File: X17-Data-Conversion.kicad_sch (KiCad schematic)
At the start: 23 parts, among them J1 Conn_01x05, J2 BG030_-_-_-_6_-_-_X_-_XXX_-_-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, J3 BG030_-_-_-_6_-_-_X_-_XXX_-_-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, SW1 1825910-6, U1 ABLS-8.000MHZ-B2-T, U2 STM32F091CCTx, U5 AZ1117IH-3.3TRG1

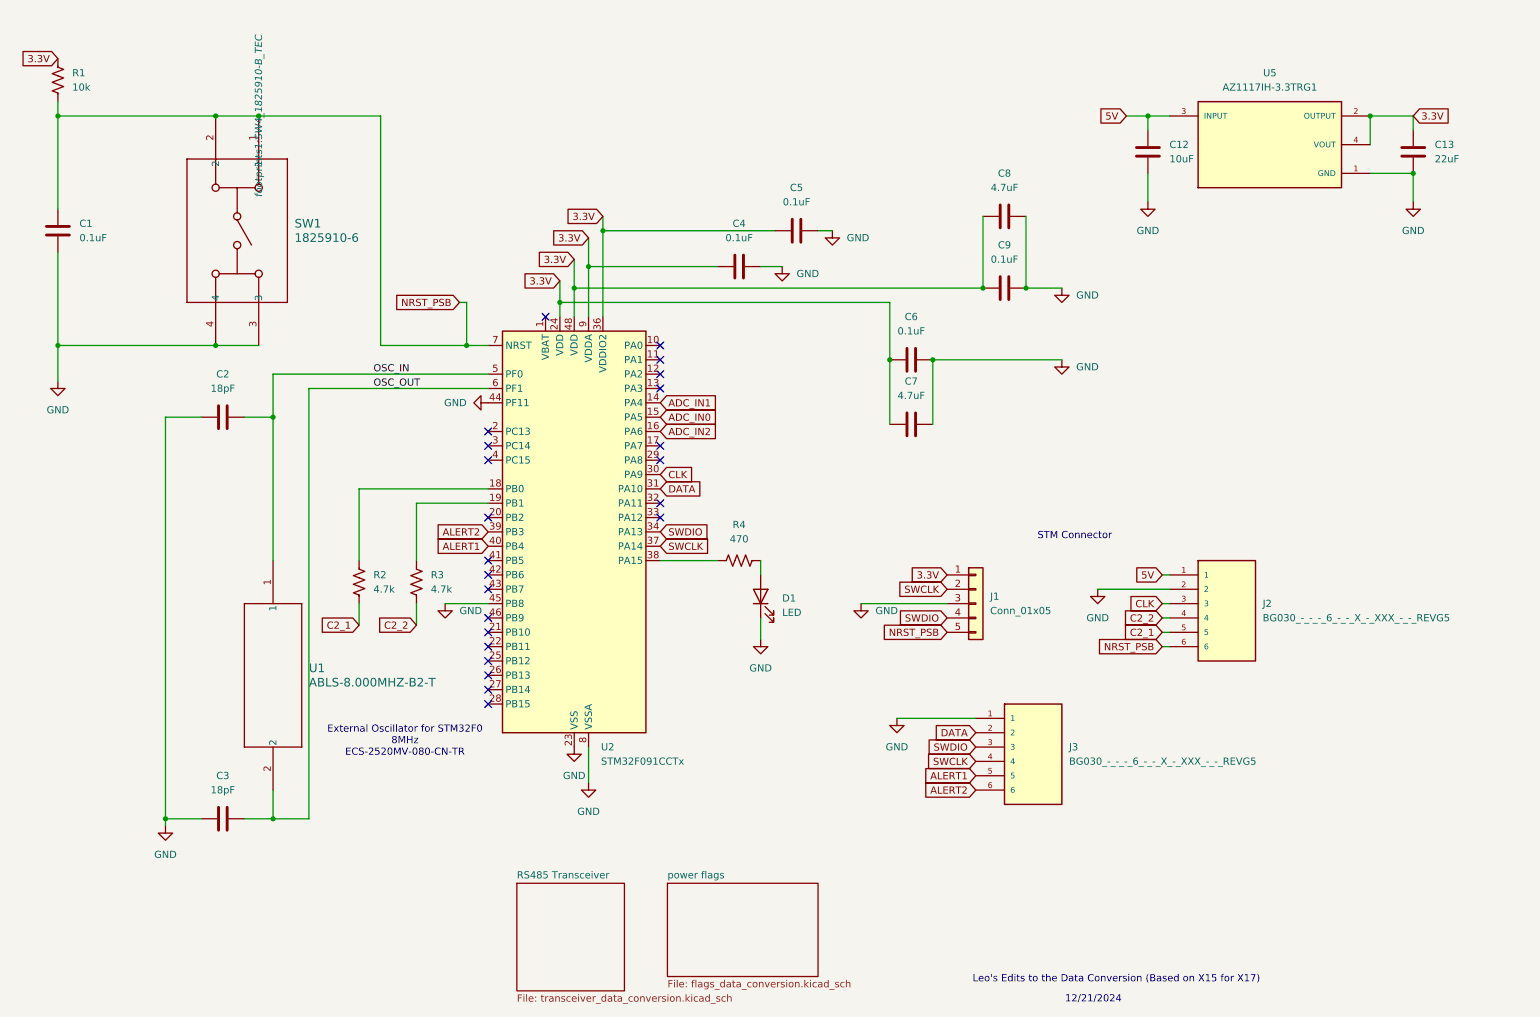
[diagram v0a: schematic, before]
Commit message: meeting today, need to rewire
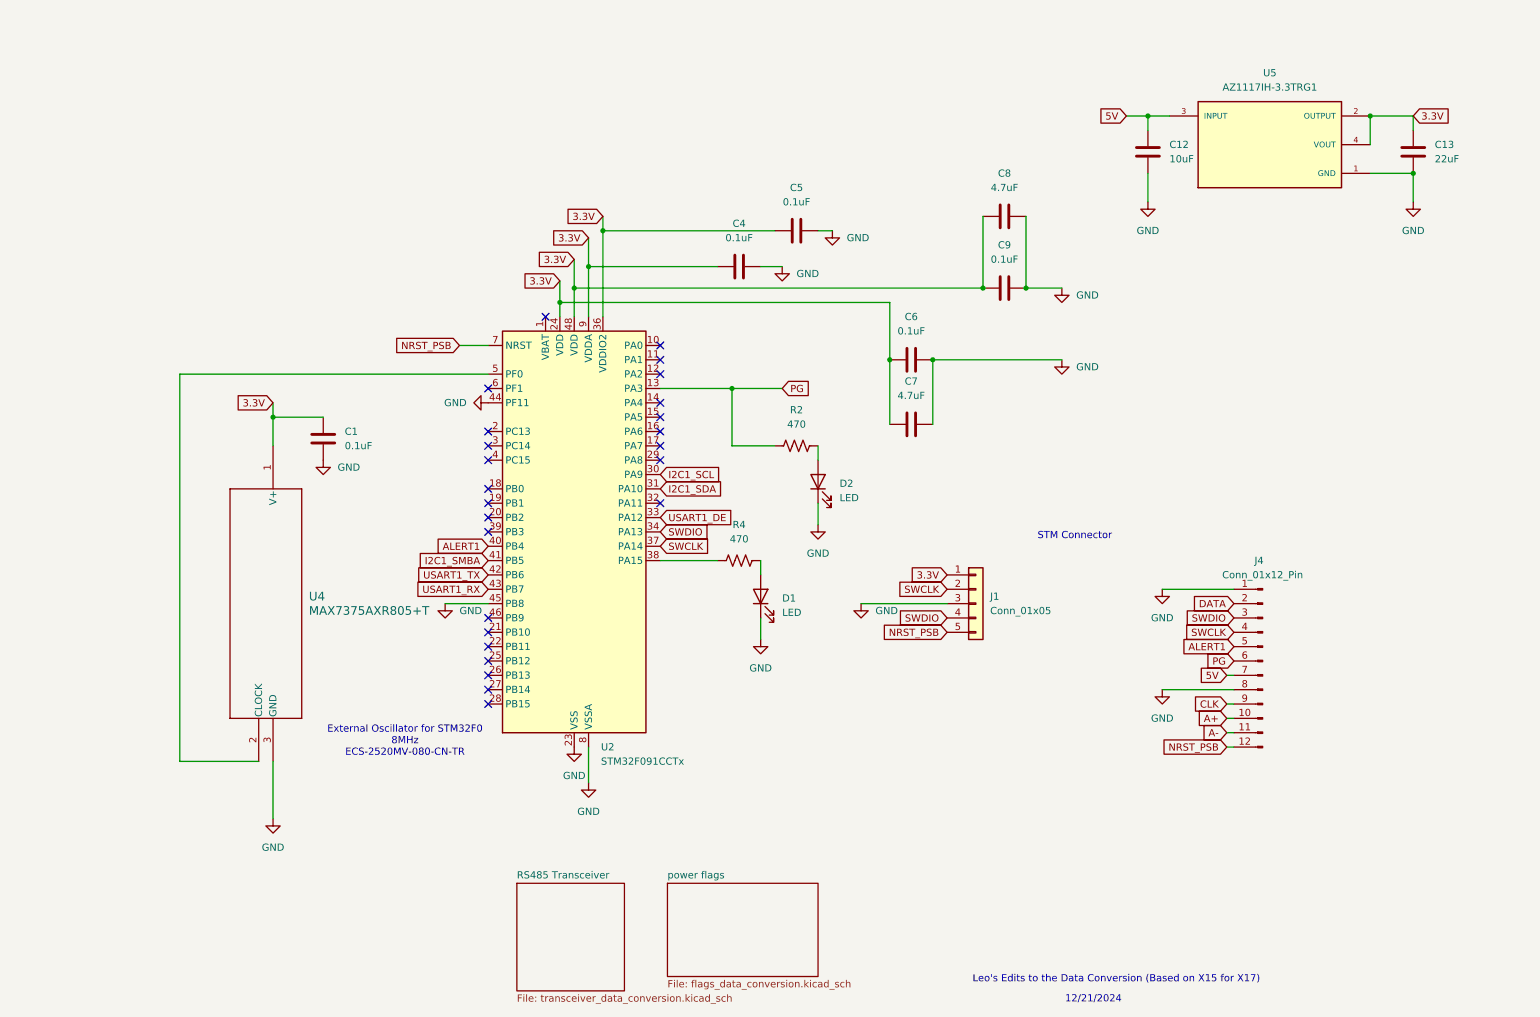
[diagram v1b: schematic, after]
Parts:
- removed C2, C3: 18pF, Capacitor_SMD:C_0603_1608Metric_Pad1.08x0.95mm_HandSolder, symbol Device:C
- removed J2, J3: BG030_-_-_-_6_-_-_X_-_XXX_-_-_REVG5, 61300611121:61300611121, symbol BG030_-_-_-_6_-_-_X_-_XXX_-_-_REVG5:BG030_-_-_-_6_-_-_X_-_XXX_-_-_REVG5
- removed R1: 10k, Resistor_SMD:R_0603_1608Metric_Pad0.98x0.95mm_HandSolder, symbol Device:R_US
- removed R3: 4.7k, Resistor_SMD:R_0603_1608Metric_Pad0.98x0.95mm_HandSolder, symbol Device:R_US
- removed SW1: 1825910-6, footprints1:SW4_1825910-B_TEC, symbol STM Switch Symbol:1825910-6
- removed U1: ABLS-8.000MHZ-B2-T, footprints2:ABLS-8.000MHZ-B2-T_ABR, symbol STM32_Oscillator:ABLS-8.000MHZ-B2-T
- added D2: LED, LED_SMD:LED_0805_2012Metric_Pad1.15x1.40mm_HandSolder, symbol Device:LED
- added J4: Conn_01x12_Pin, Library:Data Conversion two 1x6, symbol Connector:Conn_01x12_Pin
- added U4: MAX7375AXR805+T, 21-0075D_MXM, symbol 2024-12-30_21-17-45:MAX7375AXR805+T
- R2: value 4.7k -> 470
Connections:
- net 3.3V: now also C1.1, U4.1 (V+)
- net 5V: now also J4.7 (Pin_7)
- net ALERT1: now also J4.5 (Pin_5)
- net CLK: now also J4.9 (Pin_9); no longer U2.30 (PA9)
- net DATA: now also J4.2 (Pin_2); no longer U2.31 (PA10)
- net GND: now also D2.1 (K), J4.1 (Pin_1), J4.8 (Pin_8), U4.3 (GND)
- net NRST_PSB: now also J4.12 (Pin_12); no longer C1.1
- net SWCLK: now also J4.4 (Pin_4)
- net SWDIO: now also J4.3 (Pin_3)
- net PG: now reaches U2.13 (PA3)
- net PG: now also R2.1, J4.6 (Pin_6)
- net at U2.18 (PB0): no longer R2.1
- net USART1_DE: now reaches U2.33 (PA12)
- net I2C1_SMBA: now reaches U2.41 (PB5)
- net USART1_TX: now reaches U2.42 (PB6)
- net USART1_RX: now reaches U2.43 (PB7)
- net ADC_IN0: no longer names the net of U2.15 (PA5)
- net ADC_IN1: no longer names the net of U2.14 (PA4)
- net ADC_IN2: no longer names the net of U2.16 (PA6)
- net ALERT2: no longer names the net of U2.39 (PB3)
- net C2_1: no longer names the net of R2.2
- net C2_1: now also D2.2 (A)
- net OSC_IN: no longer names the net of U2.5 (PF0)
- net OSC_IN: now also U4.2 (CLOCK)
- net OSC_OUT: no longer names the net of U2.6 (PF1)
- new net A+: J4.10 (Pin_10)
- new net A-: J4.11 (Pin_11)
- new net I2C1_SCL: U2.30 (PA9)
- new net I2C1_SDA: U2.31 (PA10)
- no-connect marks 23 -> 25

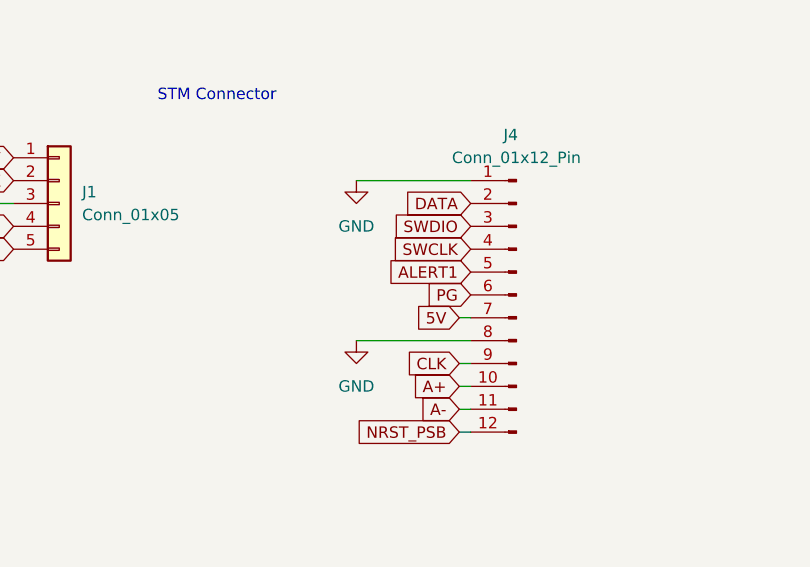
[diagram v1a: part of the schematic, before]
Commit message: hny!
lookinggood, happy new year!
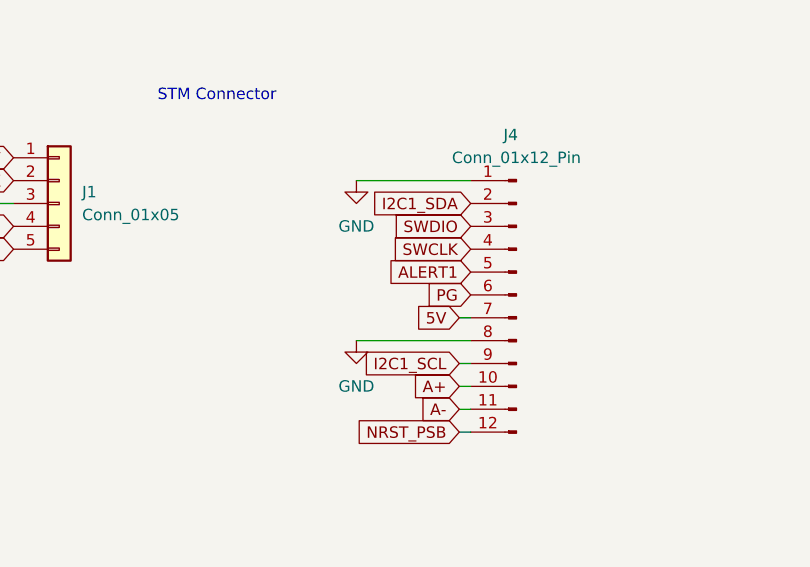
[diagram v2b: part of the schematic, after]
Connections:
- net CLK is gone; now on net I2C1_SCL: J4.9 (Pin_9)
- net DATA is gone; now on net I2C1_SDA: J4.2 (Pin_2)
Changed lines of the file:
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@@
 		)
 	)
-	(global_label "DATA"
+	(global_label "I2C1_SDA"
 		(shape input)
 		(at 238.76 123.19 180)
@@
 		)
 		(property "Intersheetrefs" "${INTERSHEET_REFS}"
-			(at 231.36 123.19 0)
+			(at 226.9453 123.19 0)
 			(effects
 				(font
@@
 		)
 	)
-	(global_label "CLK"
+	(global_label "I2C1_SCL"
 		(shape input)
 		(at 237.49 140.97 180)
@@
 		)
 		(property "Intersheetrefs" "${INTERSHEET_REFS}"
-			(at 230.9367 140.97 0)
-			(effects
-				(font
+			(at 225.7358 140.97 0)
+			(effects
+				(font

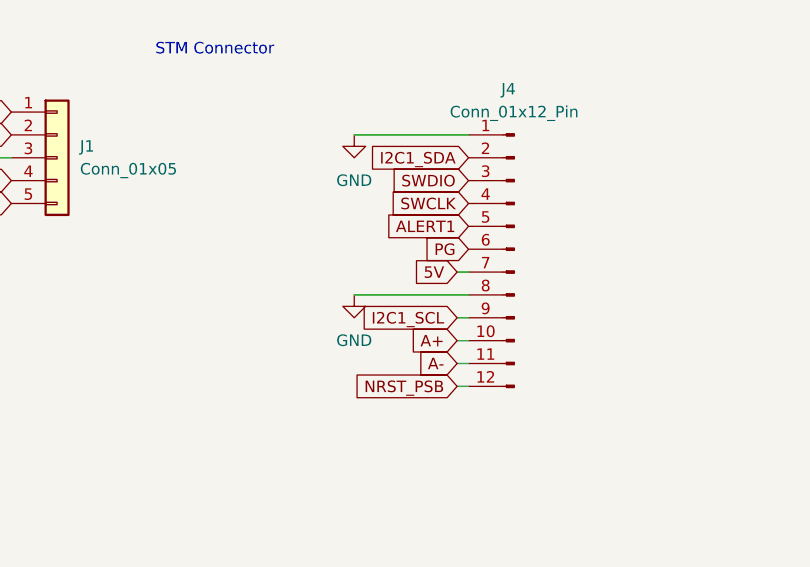
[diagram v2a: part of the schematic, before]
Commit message: daniel lookie
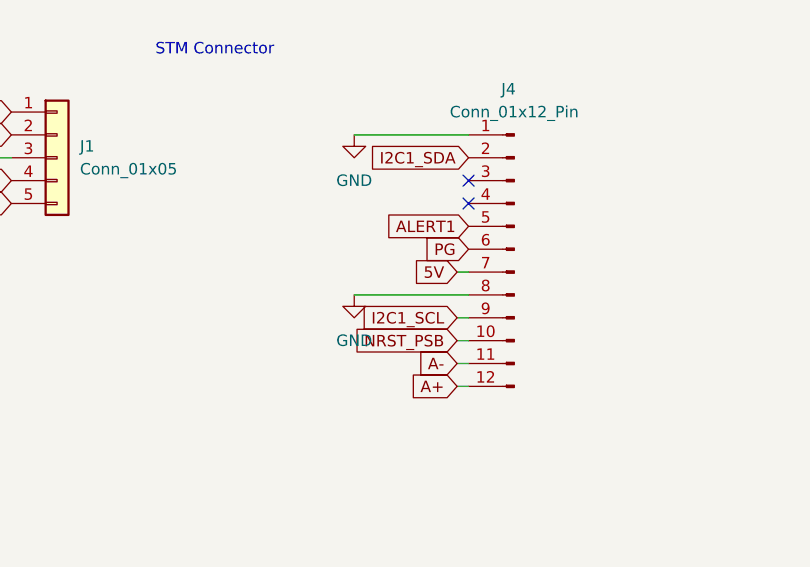
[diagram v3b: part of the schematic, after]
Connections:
- net A+: now also J4.12 (Pin_12); no longer J4.10 (Pin_10)
- net NRST_PSB: now also J4.10 (Pin_10); no longer J4.12 (Pin_12)
- net SWCLK: no longer J4.4 (Pin_4)
- net SWDIO: no longer J4.3 (Pin_3)
- no-connect marks 25 -> 27
